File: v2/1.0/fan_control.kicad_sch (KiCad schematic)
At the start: 19 parts, among them M1 Fan_4pin, M2 Fan_4pin, U1 LM2575-12BU

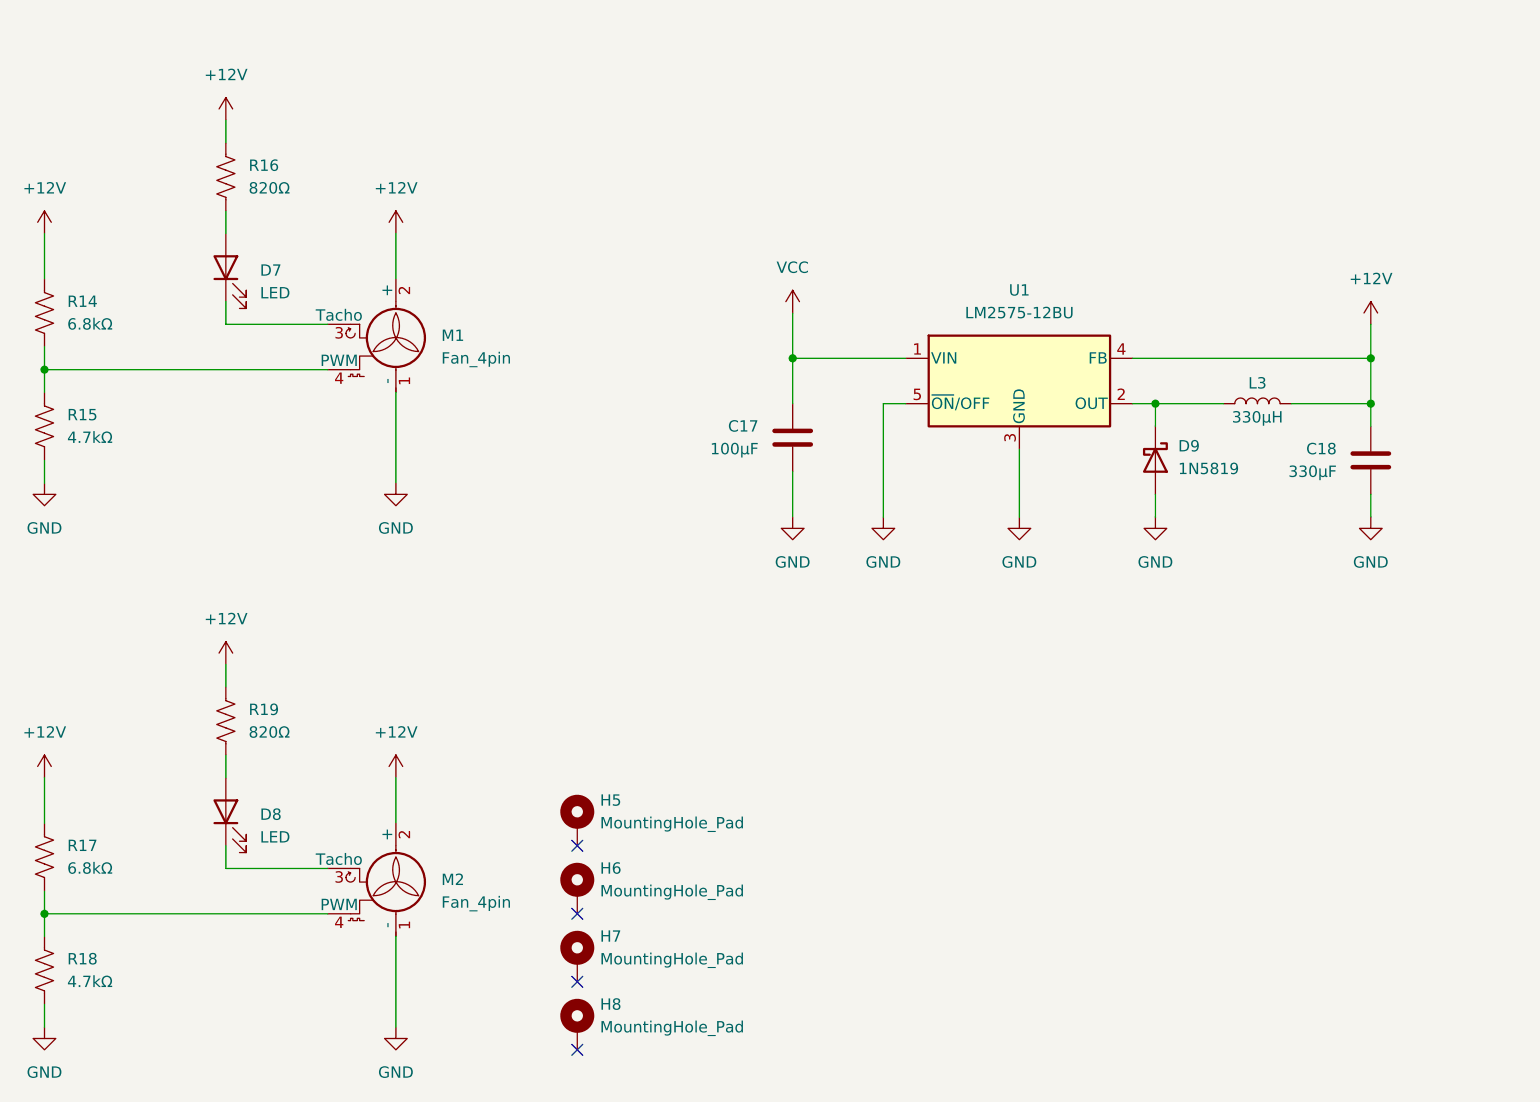
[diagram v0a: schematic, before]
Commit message: archive and update
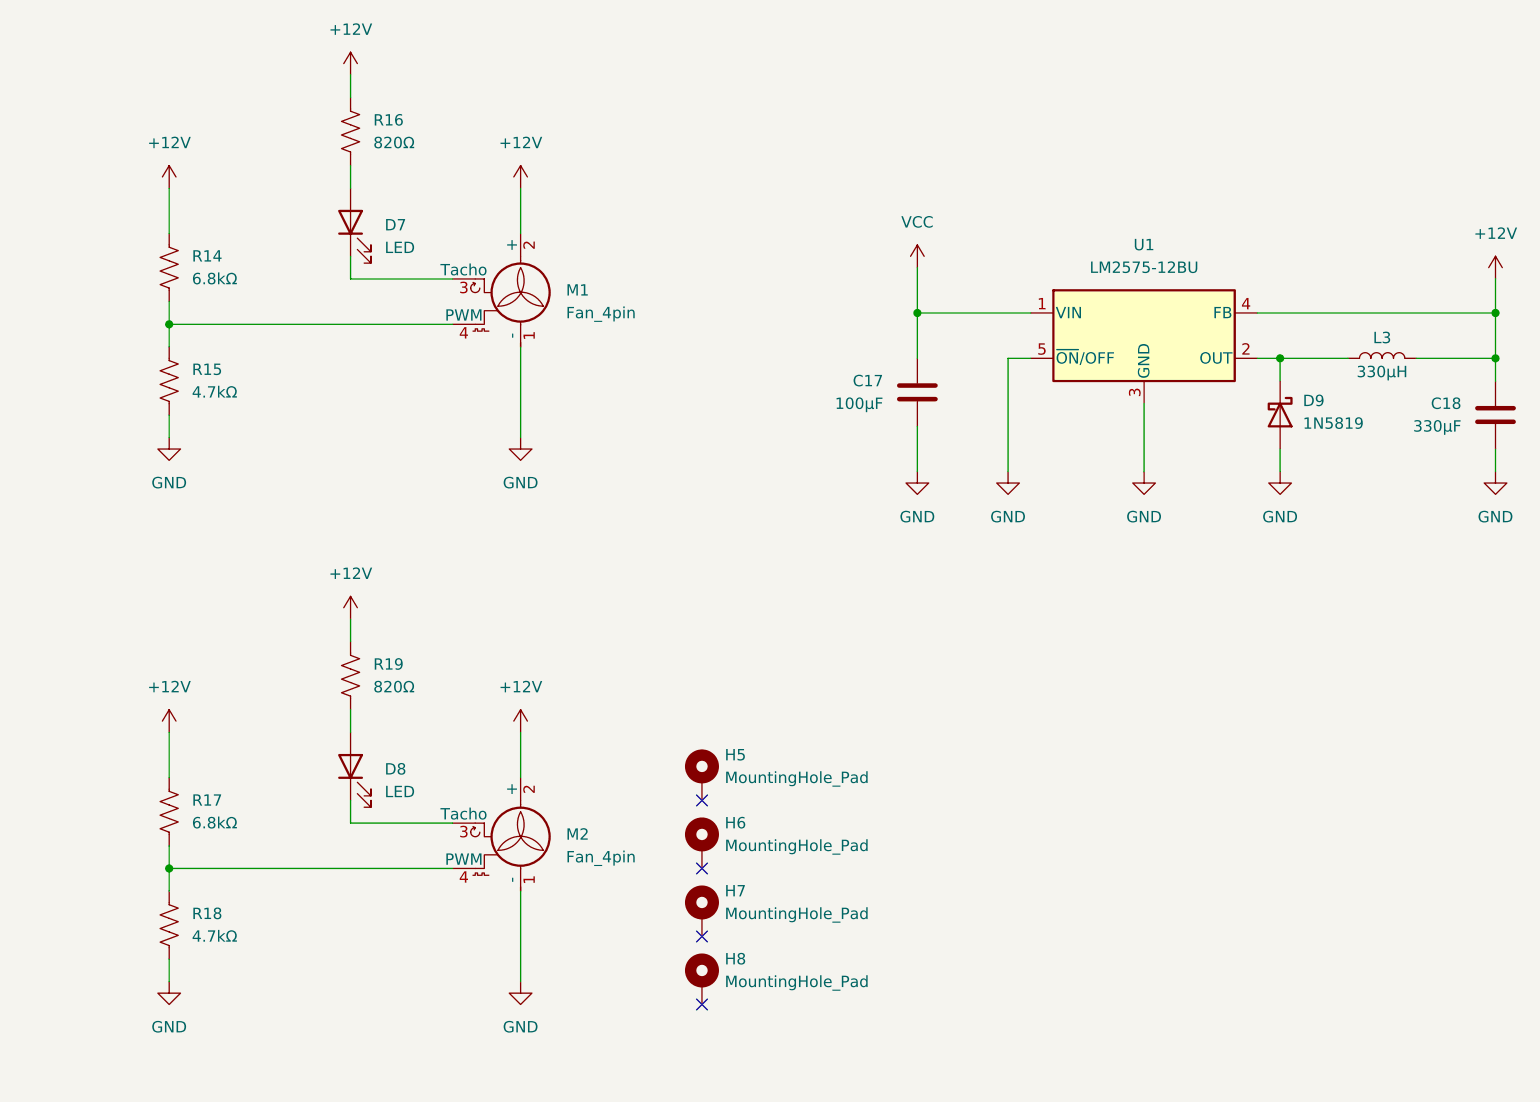
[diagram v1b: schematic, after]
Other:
- moved on the sheet: C17, C18, D7, D8, D9, H5, H6, H7, H8, L3, M1, M2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
